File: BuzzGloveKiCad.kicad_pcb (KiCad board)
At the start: 2 copper layers, 67.3 x 80.2 mm, 33 parts, among them J1 +5V, J2 8P8C, J3 GND, Q1 PN2222, Q2 PN2222, Q3 PN2222, Q4 PN2222, Q5 PN2222, Q6 PN2222

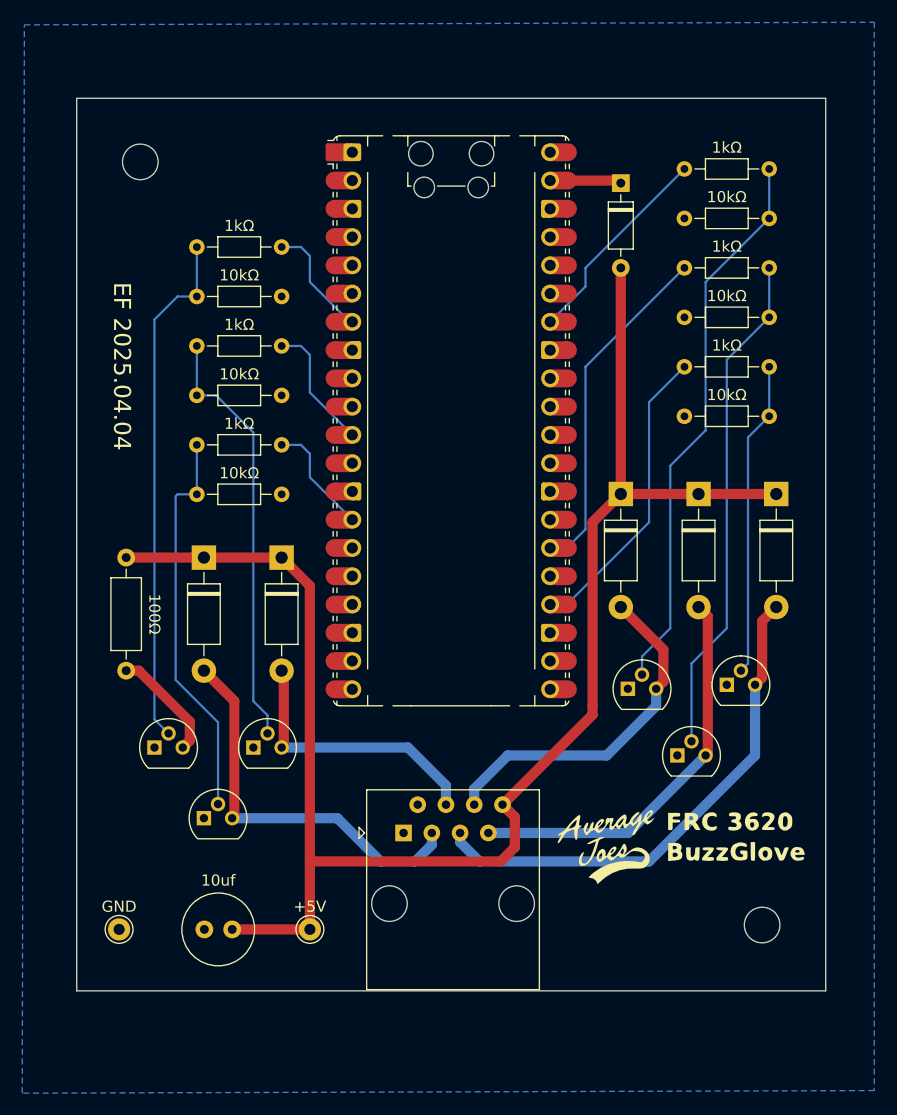
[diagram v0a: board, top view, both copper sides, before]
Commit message: Save version 25.04.14
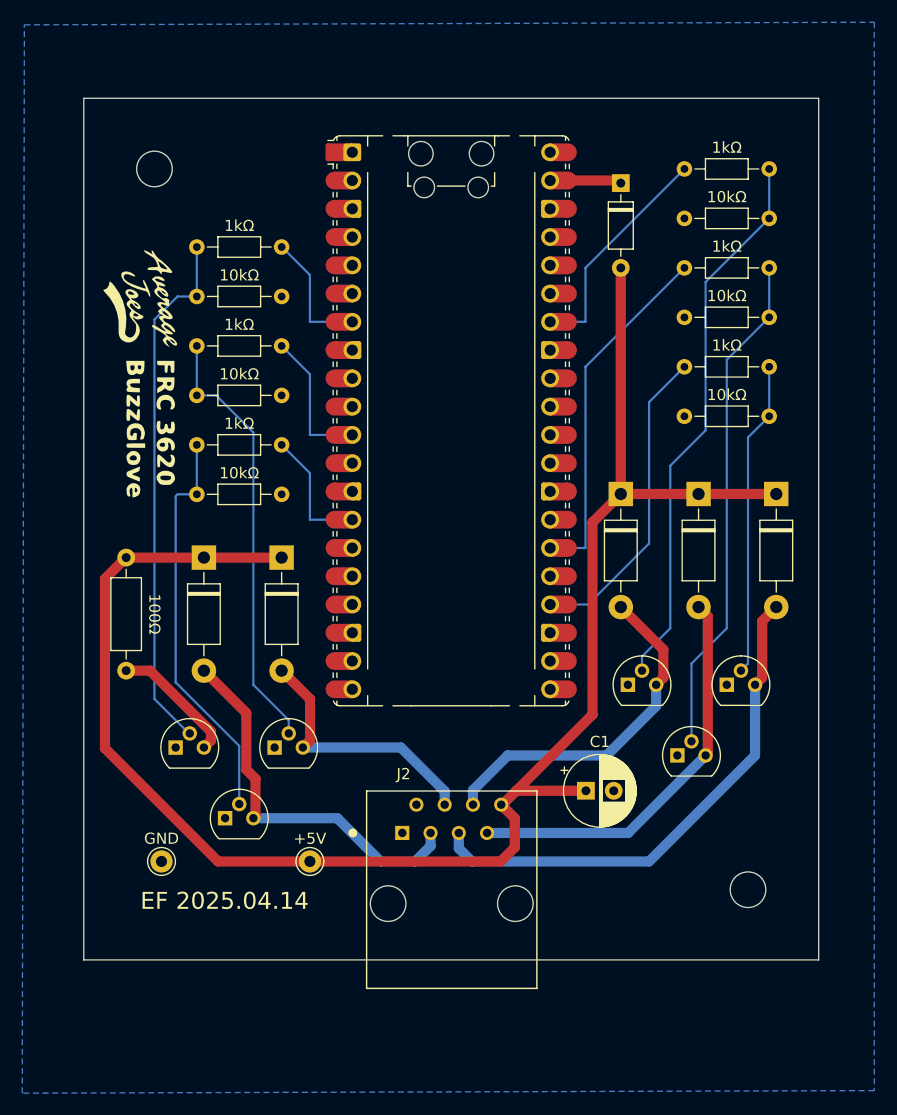
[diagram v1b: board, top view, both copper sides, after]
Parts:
- removed the REF** at (118.1, 62.9)
- removed the REF** at (174.0, 131.4)
- added REF**: MountingHole_3.2mm_M3, MountingHole:MountingHole_3.2mm_M3, F.Cu at (172.7, 128.3)
- added REF**: MountingHole_3.2mm_M3, MountingHole:MountingHole_3.2mm_M3, F.Cu at (119.4, 63.5)
- C1: footprint Capacitor_THT:C_Radial_D6.3mm_H7.0mm_P2.50mm -> Capacitor_THT:CP_Radial_D6.3mm_P2.50mm
- J2: footprint Connector_RJ:RJ45_Amphenol_54602-x08_Horizontal -> BuzzGloveFootprints:AMPHENOL_54602-908LF
- moved G*** 64.8 mm to (118.1, 83.5), turned to -90 degrees
- moved C1 34.1 mm to (158.2, 119.4), turned to 0 degrees
- moved J2 7.69 mm to (146.1, 129.5)
- moved J3 7.20 mm to (120.0, 125.7)
- moved J1 6.11 mm to (133.3, 125.7)
- moved Q4 1.91 mm to (130.2, 115.5)
- moved Q5 1.91 mm to (125.7, 121.8)
- moved Q6 1.91 mm to (121.3, 115.5)
- moved Q1 0.36 mm to (161.9, 109.9)
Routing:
- net +5V: track 145.3 -> 150.9 mm
- net X1: track 18.7 -> 20.6 mm
- net /DummyLoad: track 10.2 -> 11.6 mm
- net X5: track 10.4 -> 11.6 mm
- net X4: track 11.6 -> 12.9 mm
- net M5: track 35.7 -> 34.5 mm
- net M4: track 25.0 -> 23.8 mm
- net X3: track 27.2 -> 28.4 mm
- net X6: track 10.5 -> 11.6 mm
- net X2: track 31.0 -> 32.0 mm
- net Net-(Q6-B): track 46.8 -> 47.7 mm
- net Net-(Q5-B): track 35.7 -> 36.5 mm
- net Net-(Q4-B): track 38.5 -> 39.3 mm
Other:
- board size 67.3 x 80.2 mm -> 66 x 77.4 mm
- board text added: "EF 2025.04.14"
- board text removed: "EF 2025.04.04"
